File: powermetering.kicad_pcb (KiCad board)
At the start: 2 copper layers, 194 x 114.1 mm, 219 parts, among them J1 Conn_01x04, J10 CONN_01X02, J11 CONN_01X02, J2 Conn_01x02, J3 Conn_01x02, J4 Conn_01x02, J5 Conn_01x02, J6 HY951180A_RJ45, J7 CONN_01X02, J8 CONN_01X02, J9 CONN_01X02, P1 USB_OTG, P2 CONN_01X04, U1 KSZ8081, U10 AP1117-50, U2 ADE9000, U3 STM32F407VETx, U4 USBLC6-4SC6, U5 ALTAIR04-900, U6 AP1117-50, U7 Si8641ED-B-IS2, U8 NXE2S0505MC, Y1 Crystal, Y2 25M, Y3 RTC

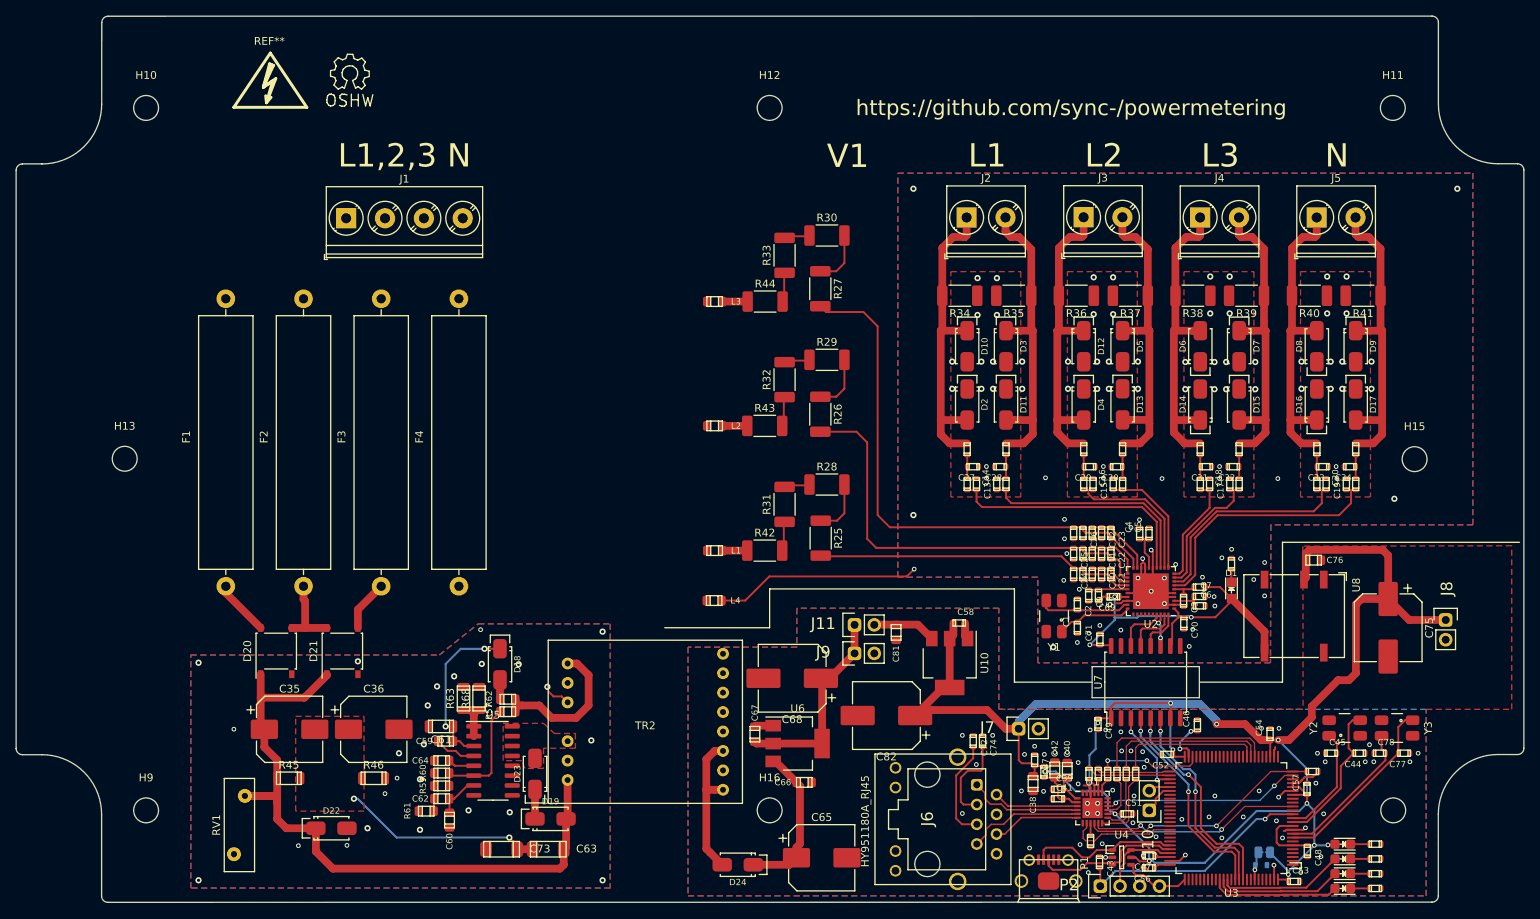
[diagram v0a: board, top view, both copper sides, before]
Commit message: V2 hardware
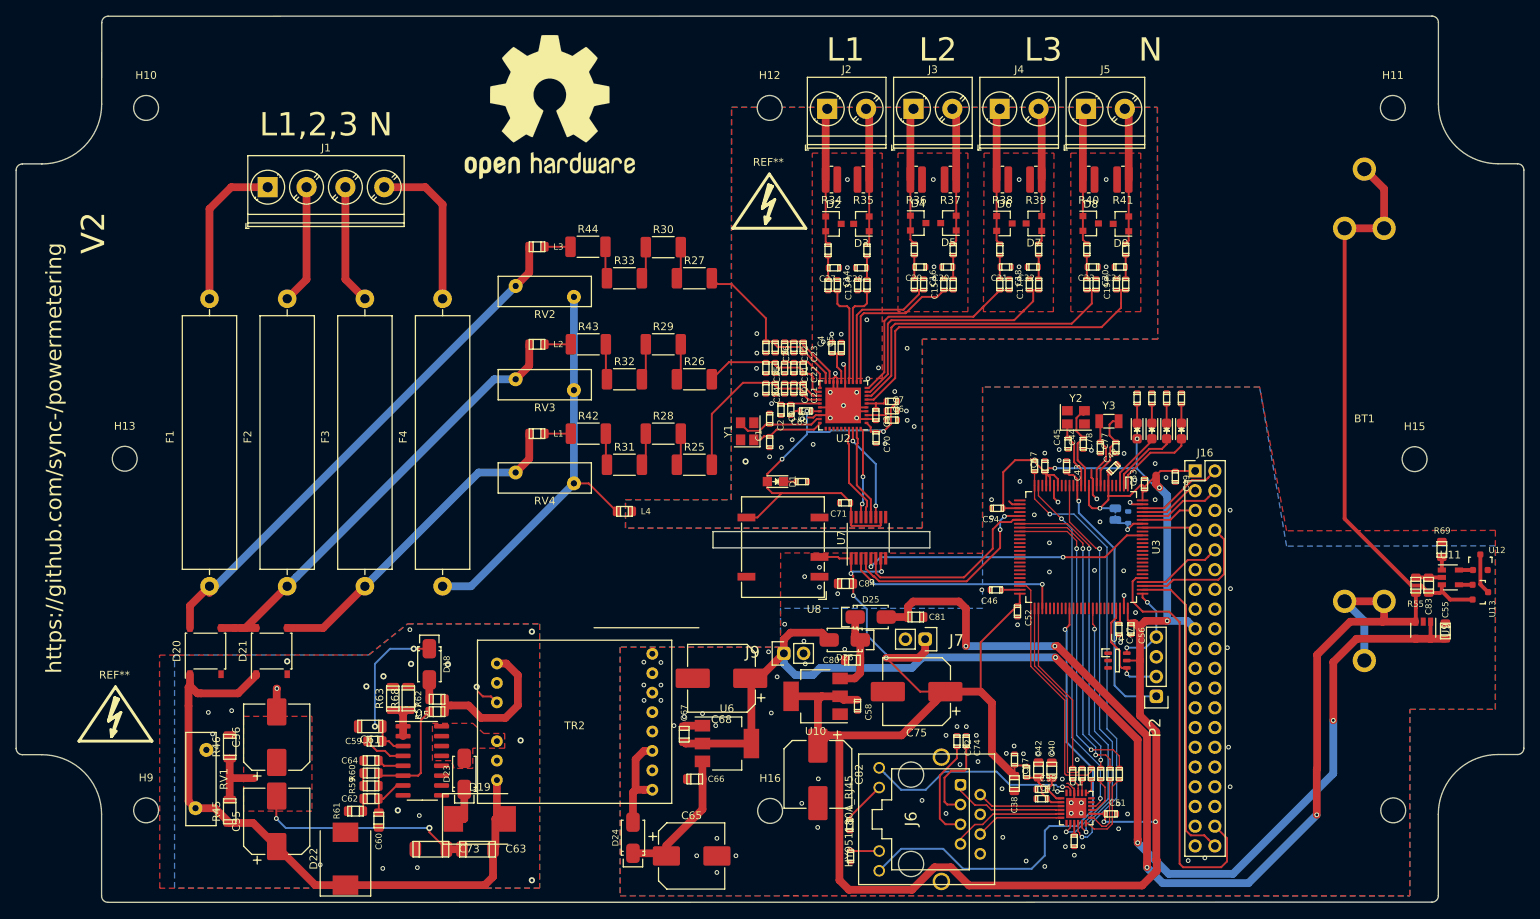
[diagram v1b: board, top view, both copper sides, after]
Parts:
- removed C76: 100n, stmbl:C_0805
- removed D10, D11, D12, D13, D14, D15, D16, D17: D, stmbl:SMA_Standard
- removed J10, J11, J8: CONN_01X02, stmbl:Pin_Header_Straight_1x02
- removed LOGO1: OPEN_HARDWARE_1, stmbl:Symbol_OSHW-Logo_SilkScreen
- removed P1: USB_OTG, stmbl:USB_Micro-B
- removed the REF** at (135.7, 61.4)
- added BT1: Battery_Cell, powermetering:18650_keystone_54, F.Cu at (276.5, 103.8)
- added C55: 1µ, stmbl:C_0805, F.Cu at (286.9, 131.6)
- added C80: 100n, stmbl:C_0805, F.Cu at (210.7, 135.3)
- added C83: 100n, stmbl:C_0805, F.Cu at (284.8, 125.7)
- added C84: 100n, stmbl:C_0805, F.Cu at (209.8, 125.5)
- added D25: D, stmbl:SMA_Standard, F.Cu at (213.0, 129.8)
- added D26: D, stmbl:SMA_Standard, F.Cu at (209.7, 132.8)
- added J16: Conn_02x20_Odd_Even, Connector_PinHeader_2.54mm:PinHeader_2x20_P2.54mm_Vertical, F.Cu at (254.8, 111.0)
- added R55: 330, stmbl:R_0805, F.Cu at (283.1, 125.7)
- added R69: 2.7k, stmbl:R_0805, F.Cu at (286.5, 121.1)
- added R70: 1k, stmbl:R_0603, F.Cu at (210.3, 156.6)
- added R71: 1k, stmbl:R_0603, F.Cu at (210.4, 160.6)
- added REF**: Symbol_HighVoltage_Type2_Top_VerySmall, stmbl:Symbol_HighVoltage_Type2_Top_VerySmall, F.Cu at (199.9, 77.0)
- added REF**: Symbol_HighVoltage_Type2_Top_VerySmall, stmbl:Symbol_HighVoltage_Type2_Top_VerySmall, F.Cu at (115.8, 143.0)
- added REF**: OSHW-Logo2_24.3x20mm_SilkScreen, Symbol:OSHW-Logo2_24.3x20mm_SilkScreen, F.Cu at (171.7, 64.2)
- added RV2: Varistor, Varistor:RV_Disc_D12mm_W3.9mm_P7.5mm, F.Cu at (167.3, 87.2)
- added RV3: Varistor, Varistor:RV_Disc_D12mm_W3.9mm_P7.5mm, F.Cu at (167.3, 99.2)
- added RV4: Varistor, Varistor:RV_Disc_D12mm_W3.9mm_P7.5mm, F.Cu at (167.3, 111.2)
- added U11: AP9101CK, Package_TO_SOT_SMD:SOT-23-5, F.Cu at (287.6, 124.7)
- added U12: NFET, stmbl:SOT-23, F.Cu at (291.4, 122.8)
- added U13: NFET, stmbl:SOT-23, F.Cu at (291.4, 126.6)
- added U9: MCP73811T-420I-OT, Package_TO_SOT_SMD:SOT-23-5, F.Cu at (284.1, 131.5)
- D19, D22: footprint stmbl:SMA_Standard -> Diode_SMD:D_SMC
- D2, D3, D4, D5, D6, D7, D8, D9: value D -> D_Schottky_x2_Serial_AKC; footprint stmbl:SMA_Standard -> Package_TO_SOT_SMD:SOT-23
- R34, R35, R36, R37, R38, R39, R40, R41: footprint Resistor_SMD:R_2010_5025Metric -> Resistor_SMD:R_0612_1632Metric
- U7: value Si8641ED-B-IS2 -> Si8641EB-B-IU; footprint Package_SO:SOIC-16W_7.5x10.3mm_P1.27mm -> Package_SO:QSOP-16_3.9x4.9mm_P0.635mm
- Y1: footprint stmbl-kicad-lib:Crystal_SMD_0603_4Pads -> Crystal:Crystal_SMD_3225-4Pin_3.2x2.5mm
- Y2: footprint stmbl:Crystal_SMD_0603_4Pads -> Crystal:Crystal_SMD_3225-4Pin_3.2x2.5mm
- Y3: footprint stmbl:Crystal_SMD_0603_4Pads -> Crystal:Crystal_SMD_3215-2Pin_3.2x1.5mm
- moved R64 67.8 mm to (253.0, 101.7), turned to 90 degrees
- moved R65 66.8 mm to (251.1, 101.7), turned to 90 degrees
- moved U8 66.4 mm to (201.7, 120.8), turned to 180 degrees
- moved R66 65.9 mm to (249.2, 101.7), turned to 90 degrees
- moved R67 65.0 mm to (247.3, 101.7), turned to 90 degrees
- moved D28 62.4 mm to (253.0, 105.9), turned to 270 degrees
- moved D29 61.3 mm to (251.1, 105.9), turned to 270 degrees
- moved C75 61.2 mm to (218.9, 139.4), turned to 180 degrees
- moved D1 60.3 mm to (200.7, 112.4), turned to 180 degrees
- moved D30 60.3 mm to (249.2, 105.9), turned to 270 degrees
- moved D31 59.4 mm to (247.3, 105.9), turned to 270 degrees
- moved R2 56.3 mm to (204.1, 112.4), turned to 0 degrees
- moved C48 55.2 mm to (244.2, 110.7), turned to 225 degrees
- moved C53 54.6 mm to (248.2, 112.7), turned to 270 degrees
- moved Y3 54.2 mm to (243.7, 104.6), turned to 0 degrees
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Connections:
- net Net-(F4-Pad2) renamed GNDS
- net Net-(U3-Pad92) renamed MMDVM_GPIO5
- D2 pad 1: N -> Net-(D2-Pad1)
- D2 pad 2: Net-(D10-Pad1) -> Net-(D2-Pad1)
- D3 pad 1: Net-(D11-Pad2) -> Net-(D3-Pad1)
- D3 pad 2: N -> Net-(D3-Pad1)
- D4 pad 1: N -> Net-(D4-Pad1)
- D4 pad 2: Net-(D12-Pad1) -> Net-(D4-Pad1)
- D5 pad 1: Net-(D13-Pad2) -> Net-(D5-Pad1)
- D5 pad 2: N -> Net-(D5-Pad1)
- D6 pad 1: N -> Net-(D6-Pad1)
- D6 pad 2: Net-(D14-Pad1) -> Net-(D6-Pad1)
- D7 pad 1: Net-(D15-Pad2) -> Net-(D7-Pad1)
- D7 pad 2: N -> Net-(D7-Pad1)
- D8 pad 1: N -> Net-(D8-Pad1)
- D8 pad 2: Net-(D16-Pad1) -> Net-(D8-Pad1)
- D9 pad 1: Net-(D17-Pad2) -> Net-(D9-Pad1)
- D9 pad 2: N -> Net-(D9-Pad1)
- J2 pad 1: Net-(D10-Pad1) -> Net-(D2-Pad1)
- J2 pad 2: Net-(D11-Pad2) -> Net-(D3-Pad1)
- J3 pad 1: Net-(D12-Pad1) -> Net-(D4-Pad1)
- J3 pad 2: Net-(D13-Pad2) -> Net-(D5-Pad1)
- J4 pad 1: Net-(D14-Pad1) -> Net-(D6-Pad1)
- J4 pad 2: Net-(D15-Pad2) -> Net-(D7-Pad1)
- J5 pad 1: Net-(D16-Pad1) -> Net-(D8-Pad1)
- J5 pad 2: Net-(D17-Pad2) -> Net-(D9-Pad1)
- J6 pad 12: Net-(J6-Pad12) -> ETH_LED
- R14 pad 2: Net-(D10-Pad1) -> Net-(D2-Pad1)
- R15 pad 2: Net-(D11-Pad2) -> Net-(D3-Pad1)
- R16 pad 2: Net-(D12-Pad1) -> Net-(D4-Pad1)
- R17 pad 2: Net-(D13-Pad2) -> Net-(D5-Pad1)
- R18 pad 2: Net-(D14-Pad1) -> Net-(D6-Pad1)
- R19 pad 2: Net-(D15-Pad2) -> Net-(D7-Pad1)
- R20 pad 2: Net-(D16-Pad1) -> Net-(D8-Pad1)
- R21 pad 2: Net-(D17-Pad2) -> Net-(D9-Pad1)
- R34 pad 2: Net-(D10-Pad1) -> Net-(D2-Pad1)
- R35 pad 1: Net-(D11-Pad2) -> Net-(D3-Pad1)
- R36 pad 2: Net-(D12-Pad1) -> Net-(D4-Pad1)
- R37 pad 1: Net-(D13-Pad2) -> Net-(D5-Pad1)
- R38 pad 2: Net-(D14-Pad1) -> Net-(D6-Pad1)
- R39 pad 1: Net-(D15-Pad2) -> Net-(D7-Pad1)
- R40 pad 2: Net-(D16-Pad1) -> Net-(D8-Pad1)
- R41 pad 1: Net-(D17-Pad2) -> Net-(D9-Pad1)
- U1 pad 23: /phy_plug/LED1K -> Net-(J6-Pad9)
- U10 pad 3: +BATT -> Net-(C80-Pad1)
- U3 pad 1: Net-(U3-Pad1) -> Net-(D28-Pad2)
- U3 pad 2: Net-(U3-Pad2) -> Net-(D29-Pad2)
- U3 pad 3: Net-(U3-Pad3) -> Net-(D30-Pad2)
- U3 pad 30: Net-(U3-Pad30) -> SCLK
- U3 pad 31: Net-(U3-Pad31) -> MISO
- U3 pad 55: USART3_TX -> Net-(U3-Pad55)
- U3 pad 56: USART3_RX -> Net-(U3-Pad56)
- U3 pad 77: Net-(U3-Pad77) -> MMDVM_NRST
- U3 pad 78: Net-(U3-Pad78) -> USART3_TX
- U3 pad 79: Net-(U3-Pad79) -> USART3_RX
- U3 pad 80: Net-(U3-Pad80) -> MMDVM_BOOT0
- U3 pad 85: Net-(D28-Pad2) -> Net-(U3-Pad85)
- U3 pad 86: Net-(D29-Pad2) -> Net-(U3-Pad86)
- U3 pad 87: Net-(D30-Pad2) -> Net-(U3-Pad87)
- U3 pad 89: SCLK -> Net-(U3-Pad89)
- U3 pad 90: MISO -> Net-(U3-Pad90)
- U3 pad 93: Net-(U3-Pad93) -> MMDVM_GPIO4
- U3 pad 95: Net-(U3-Pad95) -> MMDVM_GPIO3
- U3 pad 96: Net-(U3-Pad96) -> MMDVM_GPIO2
- U3 pad 97: Net-(U3-Pad97) -> MMDVM_GPIO1
- U3 pad 98: Net-(U3-Pad98) -> MMDVM_GPIO0
- U4 pad 4: SWCLK -> SWIO
- U4 pad 6: SWIO -> SWCLK
- U7 pad 12: Net-(U2-Pad40) -> Net-(U2-Pad39)
- U7 pad 13: Net-(U2-Pad39) -> Net-(U2-Pad37)
- U7 pad 14: Net-(U2-Pad37) -> Net-(U2-Pad40)
- Y1 pad 2: Net-(C2-Pad1) -> Net-(Y1-Pad2)
- Y1 pad 3: (no net) -> Net-(C2-Pad1)
- Y2 pad 2: Net-(C44-Pad1) -> Net-(Y2-Pad2)
- Y2 pad 3: (no net) -> Net-(C44-Pad1)
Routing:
- net +BATT: track 8.16 -> 143.6 mm, vias 0 -> 4
- net +5V: track 27.2 -> 162.3 mm, vias 0 -> 3
- net Net-(BT1-Pad2): track 0.00 -> 72.9 mm
- net ETH_LED: track 0.00 -> 62.4 mm, vias 0 -> 1
- net L1: track 7.22 -> 68.5 mm
- net MMDVM_BOOT0: track 0.00 -> 54.1 mm
- net GNDS: track 0.00 -> 53.4 mm
- net +3V3: track 264.7 -> 313.1 mm, vias 12 -> 11
- net L2: track 9.96 -> 58.3 mm
- net /UL1P: track 69.7 -> 23.1 mm
- net Net-(D13-Pad2): track 40.9 -> 0.00 mm
- net Net-(D10-Pad1): track 40.9 -> 0.00 mm
- net Net-(D11-Pad2): track 40.8 -> 0.00 mm
- net Net-(D17-Pad2): track 40.8 -> 0.00 mm
- net Net-(D12-Pad1): track 40.8 -> 0.00 mm
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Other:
- outline, holes or cut-outs redrawn
- board text added: "V2"
- board text removed: "V1"
